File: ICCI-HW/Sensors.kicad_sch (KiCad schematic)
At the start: 19 parts

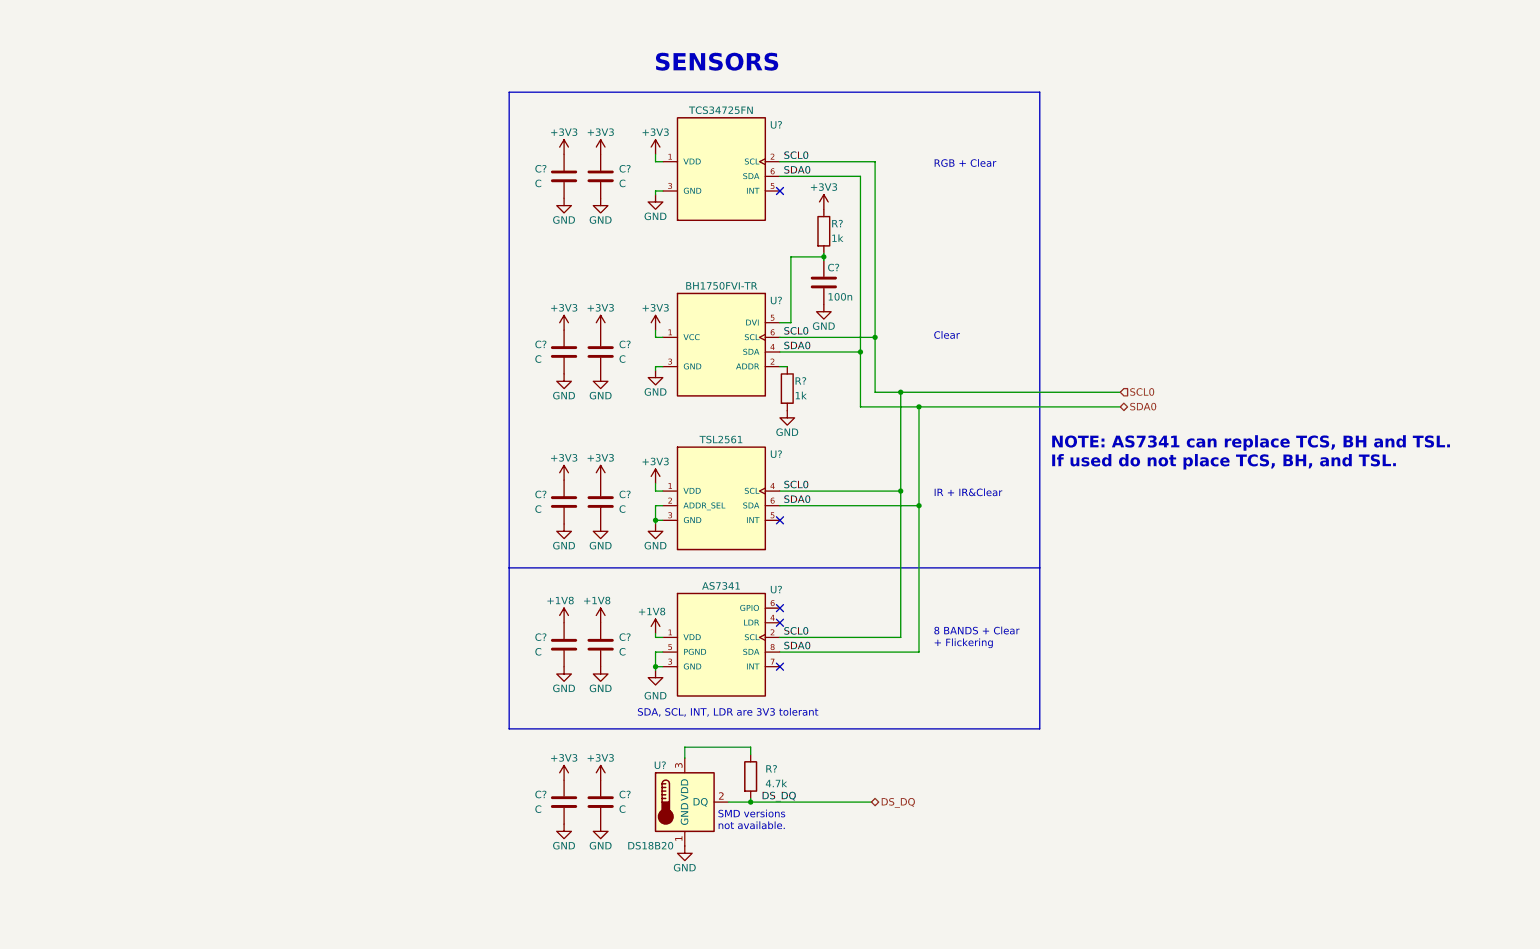
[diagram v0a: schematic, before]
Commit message: updated
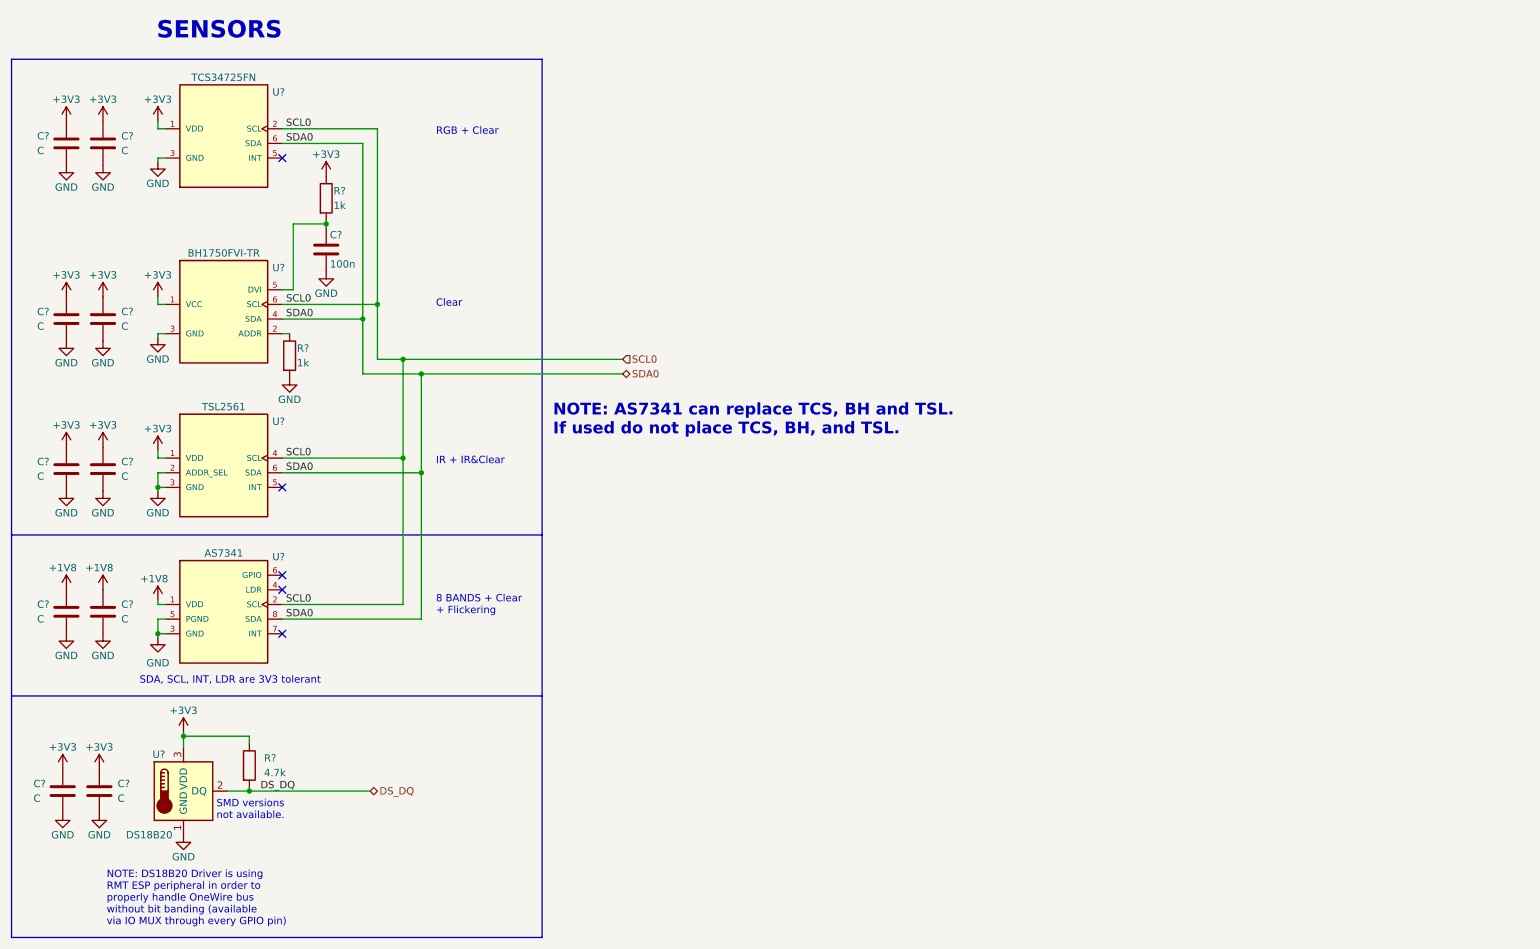
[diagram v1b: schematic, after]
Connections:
- net +3V3: now also R?.1, U?.3 (VDD)
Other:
- note added: "NOTE: DS18B20 Driver is using RMT ESP peripheral in order to properly handle OneWire bus without bit banding (available via IO MUX through every GPIO pin)"
- moved on the sheet: C?, R?, U?
